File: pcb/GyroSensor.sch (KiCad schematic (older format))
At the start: 2 parts, among them J6 GyroLeft, J7 GyroRight

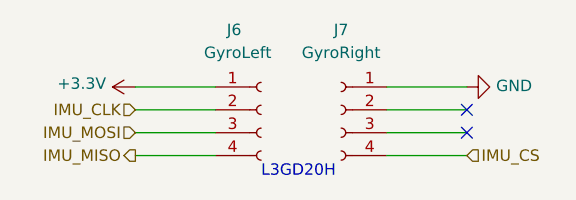
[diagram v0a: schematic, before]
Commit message: Update schematic
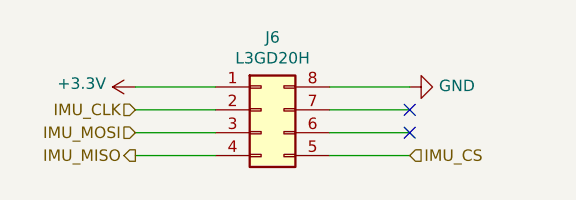
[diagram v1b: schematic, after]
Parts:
- removed J6: GyroLeft, Pin_Headers:Pin_Header_Straight_1x04_Pitch2.54mm, symbol Connector:Conn_01x04_Female
- removed J7: GyroRight, Pin_Headers:Pin_Header_Straight_1x04_Pitch2.54mm, symbol Connector:Conn_01x04_Female
- added J6: L3GD20H, Zero_Module:L3GD20HBoard, symbol Connector_Generic:Conn_02x04_Counter_Clockwise
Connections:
- net +3V3: now also J6.1 (Pin_1)
- net GND: now also J6.8 (Pin_8)
- net IMU_CLK: now also J6.2 (Pin_2)
- net IMU_CS: now also J6.5 (Pin_5)
- net IMU_MISO: now also J6.4 (Pin_4)
- net IMU_MOSI: now also J6.3 (Pin_3)
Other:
- note removed: "L3GD20H"
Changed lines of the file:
@@
 $EndDescr
-$Comp
-L Connector:Conn_01x04_Female J6
-U 1 1 61641C2F
-P 3050 1800
-F 0 "J6" H 2900 2150 50  0000 L CNN
-F 1 "GyroLeft" H 2800 2050 50  0000 L CNN
-F 2 "Pin_Headers:Pin_Header_Straight_1x04_Pitch2.54mm" H 3050 1800 50  0001 C CNN
-F 3 "~" H 3050 1800 50  0001 C CNN
-	1    3050 1800
-	1    0    0    -1
-$EndComp
-$Comp
-L Connector:Conn_01x04_Female J7
-U 1 1 61643819
-P 3400 1800
-F 0 "J7" H 3400 2150 50  0000 C CNN
-F 1 "GyroRight" H 3400 2050 50  0000 C CNN
-F 2 "Pin_Headers:Pin_Header_Straight_1x04_Pitch2.54mm" H 3400 1800 50  0001 C CNN
-F 3 "~" H 3400 1800 50  0001 C CNN
-	1    3400 1800
-	-1   0    0    -1
-$EndComp
 $Comp
 L power:+3.3V #PWR0114
@@
 	2500 2000 2850 2000
 Wire Wire Line
-	3600 1700 3950 1700
+	3350 1700 3700 1700
 Wire Wire Line
-	3600 1800 3950 1800
+	3350 1800 3700 1800
 Wire Wire Line
-	3600 1900 3950 1900
+	3350 1900 3700 1900
 Wire Wire Line
-	3600 2000 3950 2000
+	3350 2000 3700 2000
 Text HLabel 2500 2000 0    50   Output ~ 0
 IMU_MISO
-Text HLabel 3950 2000 2    50   Input ~ 0
+Text HLabel 3700 2000 2    50   Input ~ 0
 IMU_CS
 $Comp
 L power:GND #PWR0122
 U 1 1 6164A75A
-P 3950 1700
-F 0 "#PWR0122" H 3950 1450 50  0001 C CNN
-F 1 "GND" V 3955 1572 50  0000 R CNN
-F 2 "" H 3950 1700 50  0001 C CNN
-F 3 "" H 3950 1700 50  0001 C CNN
-	1    3950 1700
+P 3700 1700
+F 0 "#PWR0122" H 3700 1450 50  0001 C CNN
+F 1 "GND" V 3705 1572 50  0000 R CNN
+F 2 "" H 3700 1700 50  0001 C CNN
+F 3 "" H 3700 1700 50  0001 C CNN
+	1    3700 1700
 	0    -1   -1   0
 $EndComp
-NoConn ~ 3950 1800
-NoConn ~ 3950 1900
+NoConn ~ 3700 1800
+NoConn ~ 3700 1900
 Text HLabel 2500 1900 0    50   Input ~ 0
 IMU_MOSI
-Text Notes 3050 2100 0    50   ~ 0
-L3GD20H
+$Comp
+L Connector_Generic:Conn_02x04_Counter_Clockwise J6
+U 1 1 6171D7CB
+P 3050 1800
+F 0 "J6" H 3100 2117 50  0000 C CNN
+F 1 "L3GD20H" H 3100 2026 50  0000 C CNN
+F 2 "Zero_Module:L3GD20HBoard" H 3050 1800 50  0001 C CNN
+F 3 "~" H 3050 1800 50  0001 C CNN
+	1    3050 1800
+	1    0    0    -1
+$EndComp
 $EndSCHEMATC

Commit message: Write about where to buy the parts
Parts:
- J6: Buy (none) -> https://akizukidenshi.com/catalog/g/gK-15096/; Vendor (none) -> https://akizukidenshi.com/catalog/g/gK-15096/
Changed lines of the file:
@@
 F 1 "L3GD20H" H 3100 2026 50  0000 C CNN
 F 2 "Zero_Module:L3GD20HBoard" H 3050 1800 50  0001 C CNN
-F 3 "~" H 3050 1800 50  0001 C CNN
+F 3 "https://akizukidenshi.com/catalog/g/gK-15096/" H 3050 1800 50  0001 C CNN
+F 4 "https://akizukidenshi.com/catalog/g/gK-15096/" H 3050 1800 50  0001 C CNN "Buy"
+F 5 "https://akizukidenshi.com/catalog/g/gK-15096/" H 3050 1800 50  0001 C CNN "Vendor"
 	1    3050 1800
 	1    0    0    -1
